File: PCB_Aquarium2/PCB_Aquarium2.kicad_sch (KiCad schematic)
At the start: 38 parts, among them J1 Conn_02x20_Counter_Clockwise, J10 Conn_01x03, J11 Conn_01x03, J12 Conn_01x03, J13 Conn_01x03, J14 Conn_01x03, J15 Conn_01x03, J16 Conn_01x03, J17 Conn_01x03, J18 Conn_01x03, J19 Conn_01x03, J2 Conn_01x03, J20 Conn_01x03, J21 Conn_01x03, J22 Conn_01x03, J23 Conn_01x03, J24 Conn_01x03, J25 Conn_01x03, J26 Conn_01x03, J27 Conn_01x04, J28 Conn_01x03, J29 Conn_01x03, J3 Conn_01x03, J30 Conn_01x03, J31 Conn_01x03, J32 Conn_01x03, J33 Conn_01x03, J34 Conn_01x03, J35 Conn_01x03, J36 Conn_01x03, J37 Conn_01x03, J4 Conn_01x03, J5 Conn_01x03, J6 Conn_01x03, J7 Conn_ST_STDC14, J8 Conn_01x02, J9 Conn_01x03, U1 STM32G431KBTx

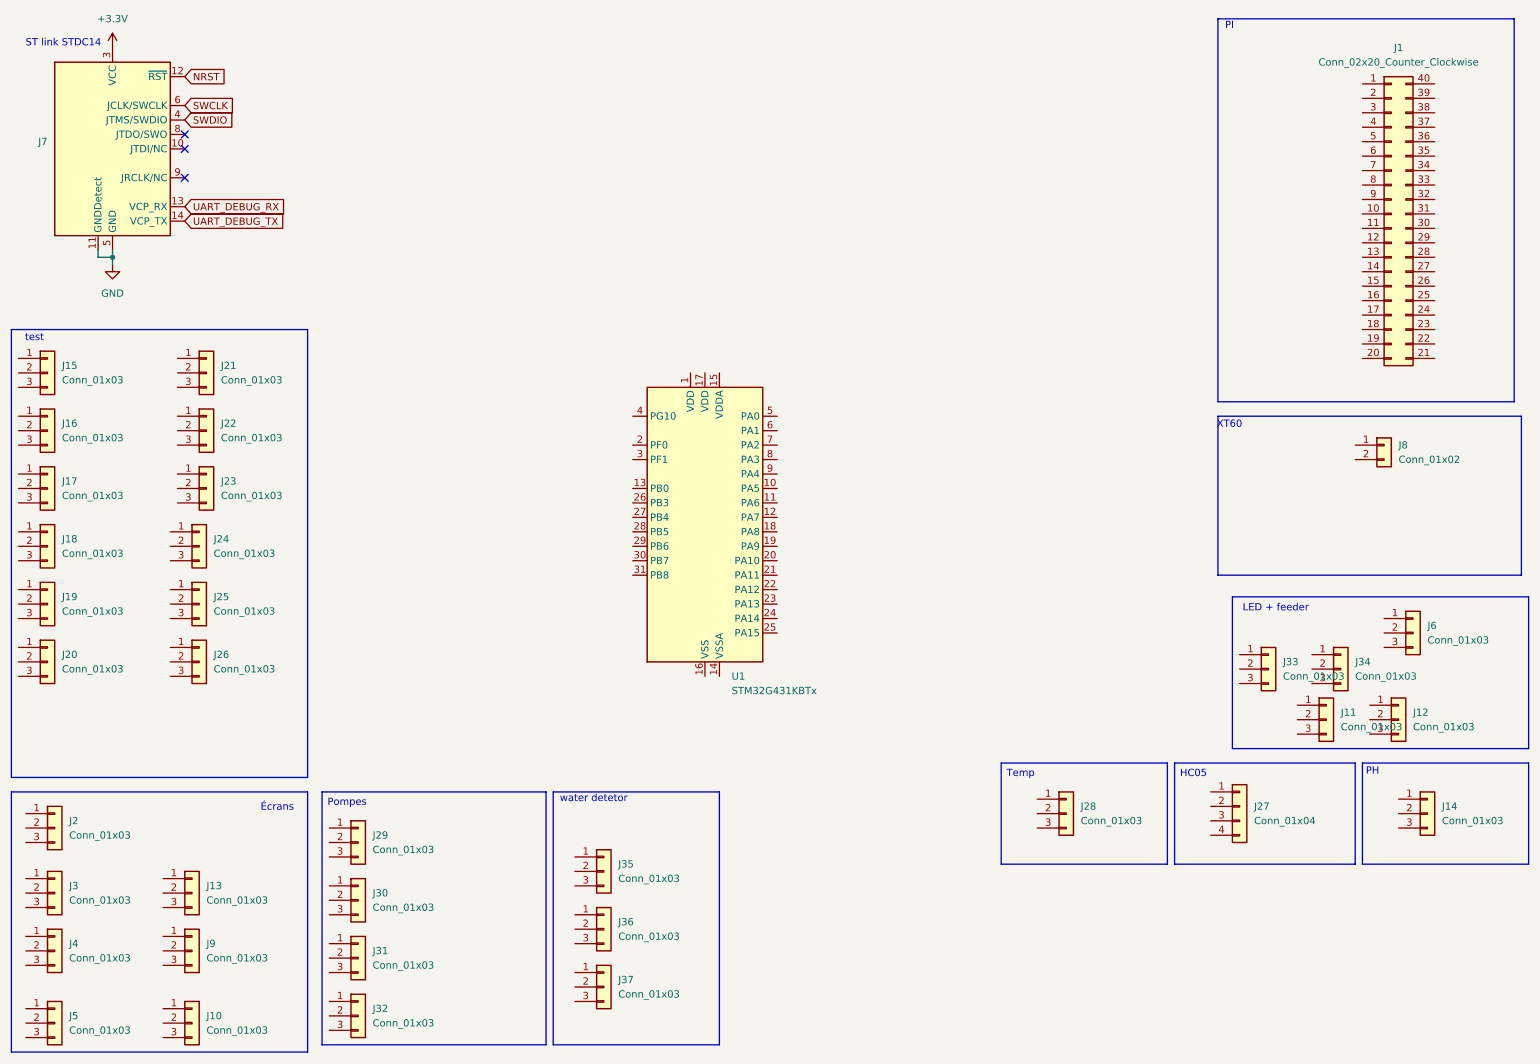
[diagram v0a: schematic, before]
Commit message: PCB-v0
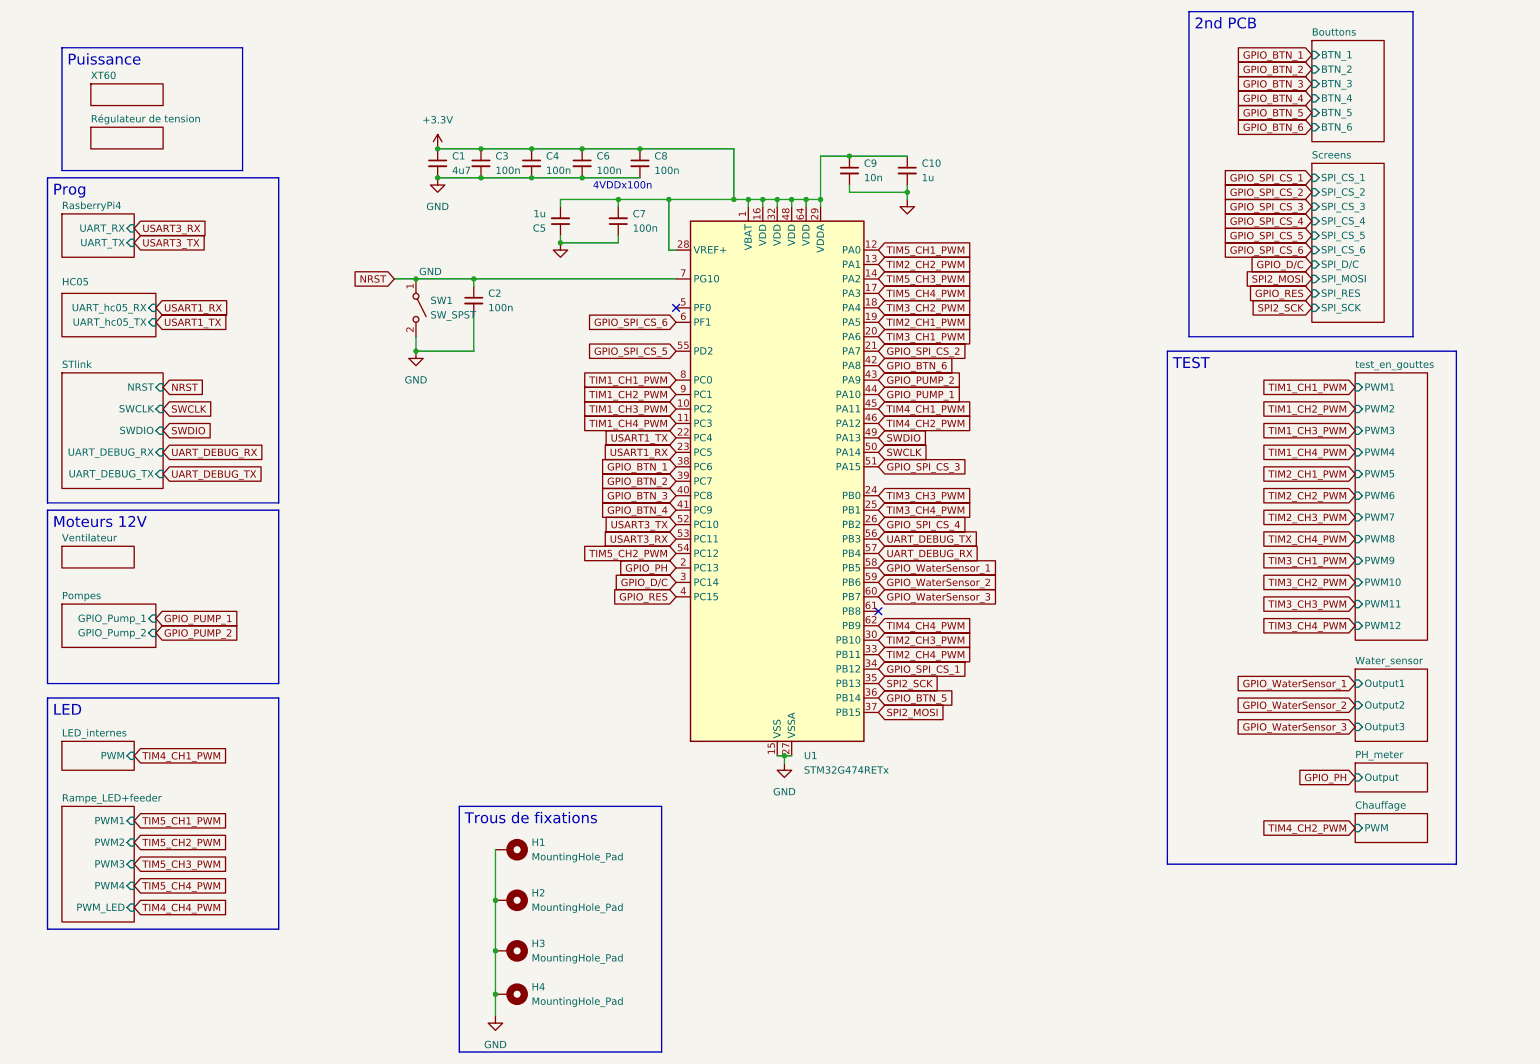
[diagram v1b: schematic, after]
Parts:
- removed J1: Conn_02x20_Counter_Clockwise, Connector_PinSocket_2.54mm:PinSocket_2x20_P2.54mm_Vertical, symbol Connector_Generic:Conn_02x20_Counter_Clockwise
- removed J10, J11, J12, J13, J14, J15, J16, J17, J18, J19, J2, J20, J21, J22, J23, J24, J25, J26, J28, J29, J3, J30, J31, J32, J33, J34, J35, J36, J37, J4, J5, J6, J9: Conn_01x03, Connector_JST:JST_EH_B3B-EH-A_1x03_P2.50mm_Vertical, symbol Connector_Generic:Conn_01x03
- removed J27: Conn_01x04, Connector_JST:JST_EH_B4B-EH-A_1x04_P2.50mm_Vertical, symbol Connector_Generic:Conn_01x04
- removed J7: Conn_ST_STDC14, Connector_PinHeader_1.27mm:PinHeader_2x07_P1.27mm_Vertical_SMD, symbol Connector:Conn_ST_STDC14
- removed J8: Conn_01x02, Connector_JST:JST_EH_B2B-EH-A_1x02_P2.50mm_Vertical, symbol Connector_Generic:Conn_01x02
- removed U1: STM32G431KBTx, Package_QFP:LQFP-32_7x7mm_P0.8mm, symbol MCU_ST_STM32G4:STM32G431KBTx
- added C1: 4u7, Capacitor_SMD:C_0402_1005Metric, symbol Device:C_Small
- added C10, C5: 1u, Capacitor_SMD:C_0402_1005Metric, symbol Device:C_Small
- added C2, C3, C4, C6, C7, C8: 100n, Capacitor_SMD:C_0402_1005Metric, symbol Device:C_Small
- added C9: 10n, Capacitor_SMD:C_0402_1005Metric, symbol Device:C_Small
- added H1, H2, H3, H4: MountingHole_Pad, MountingHole:MountingHole_3.2mm_M3_Pad_Via, symbol Mechanical:MountingHole_Pad
- added SW1: SW_SPST, mylib:SW_Push_1P1T_NO_6x6mm_H9.5mm, symbol Switch:SW_SPST
- added U1: STM32G474RETx, Package_QFP:LQFP-64_10x10mm_P0.5mm, symbol MCU_ST_STM32G4:STM32G474RETx
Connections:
- net +3.3V: now also C1.1, C10.1, C3.1, C4.1, C5.2, C6.1, C7.2, C8.1, C9.1, U1.1 (VBAT), U1.16 (VDD), U1.28 (VREF+), U1.29 (VDDA), U1.32 (VDD), U1.48 (VDD), U1.64 (VDD)
- net GND: now also C1.2, C10.2, C2.2, C3.2, C4.2, C5.1, C6.2, C7.1, C8.2, C9.2, H1.1, H2.1, H3.1, H4.1, SW1.2 (B), U1.15 (VSS), U1.27 (VSSA), U1.31 (VSS), U1.47 (VSS), U1.63 (VSS)
- net NRST: now also C2.1, SW1.1 (A), U1.7 (PG10)
- net SWCLK: now also U1.50 (PA14)
- net SWDIO: now also U1.49 (PA13)
- net UART_DEBUG_RX: now also U1.57 (PB4)
- net UART_DEBUG_TX: now also U1.56 (PB3)
- new net GPIO_BTN_1: U1.38 (PC6)
- new net GPIO_BTN_2: U1.39 (PC7)
- new net GPIO_BTN_3: U1.40 (PC8)
- new net GPIO_BTN_4: U1.41 (PC9)
- new net GPIO_BTN_5: U1.36 (PB14)
- new net GPIO_BTN_6: U1.42 (PA8)
- new net GPIO_D/C: U1.3 (PC14)
- new net GPIO_PH: U1.2 (PC13)
- new net GPIO_PUMP_1: U1.44 (PA10)
- new net GPIO_PUMP_2: U1.43 (PA9)
- new net GPIO_RES: U1.4 (PC15)
- new net GPIO_SPI_CS_1: U1.34 (PB12)
- new net GPIO_SPI_CS_2: U1.21 (PA7)
- new net GPIO_SPI_CS_3: U1.51 (PA15)
- new net GPIO_SPI_CS_4: U1.26 (PB2)
- new net GPIO_SPI_CS_5: U1.55 (PD2)
- new net GPIO_SPI_CS_6: U1.6 (PF1)
- new net GPIO_WaterSensor_1: U1.58 (PB5)
- new net GPIO_WaterSensor_2: U1.59 (PB6)
- new net GPIO_WaterSensor_3: U1.60 (PB7)
- new net SPI2_MOSI: U1.37 (PB15)
- new net SPI2_SCK: U1.35 (PB13)
- new net TIM1_CH1_PWM: U1.8 (PC0)
- new net TIM1_CH2_PWM: U1.9 (PC1)
- new net TIM1_CH3_PWM: U1.10 (PC2)
- new net TIM1_CH4_PWM: U1.11 (PC3)
- new net TIM2_CH1_PWM: U1.19 (PA5)
- new net TIM2_CH2_PWM: U1.13 (PA1)
- new net TIM2_CH3_PWM: U1.30 (PB10)
- new net TIM2_CH4_PWM: U1.33 (PB11)
- new net TIM3_CH1_PWM: U1.20 (PA6)
- new net TIM3_CH2_PWM: U1.18 (PA4)
- new net TIM3_CH3_PWM: U1.24 (PB0)
- new net TIM3_CH4_PWM: U1.25 (PB1)
- new net TIM4_CH1_PWM: U1.45 (PA11)
- new net TIM4_CH2_PWM: U1.46 (PA12)
- new net TIM4_CH4_PWM: U1.62 (PB9)
- new net TIM5_CH1_PWM: U1.12 (PA0)
- new net TIM5_CH2_PWM: U1.54 (PC12)
- new net TIM5_CH3_PWM: U1.14 (PA2)
- new net TIM5_CH4_PWM: U1.17 (PA3)
- new net USART1_RX: U1.23 (PC5)
- new net USART1_TX: U1.22 (PC4)
- new net USART3_RX: U1.53 (PC11)
- new net USART3_TX: U1.52 (PC10)
- no-connect marks 3 -> 2
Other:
- added sheet Bouttons (Bouttons_connecteurs.kicad_sch)
- added sheet Chauffage (Chauffage.kicad_sch)
- added sheet HC05 (HC05.kicad_sch)
- added sheet LED_internes (LED_internes.kicad_sch)
- added sheet PH_meter (PH_meter.kicad_sch)
- added sheet Pompes (Pompes.kicad_sch)
- added sheet Rampe_LED+feeder (Rampe_LED+feeder.kicad_sch)
- added sheet RasberryPi4 (RasberryPi4.kicad_sch)
- added sheet Régulateur de tension (Régulateur_de_tension.kicad_sch)
- added sheet STlink (STlink.kicad_sch)
- added sheet Screens (screens_bouttons.kicad_sch)
- added sheet Ventilateur (Ventialteur.kicad_sch)
- added sheet Water_sensor (Water_sensor.kicad_sch)
- added sheet XT60 (XT60.kicad_sch)
- added sheet test_en_gouttes (test_en_gouttes.kicad_sch)
- note added: "4VDDx100n"
- note removed: "LED + feeder"
- note removed: "PH"
- note removed: "PI"
- note removed: "ST link STDC14"
- note removed: "XT60"
- note removed: "test"
- note removed: "water detetor"
- note removed: "Écrans"
